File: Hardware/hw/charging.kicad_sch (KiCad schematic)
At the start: 22 parts, among them J1 Screw_Terminal_01x02, J2 Screw_Terminal_01x02, J3 Conn_01x05_Pin, J5 Conn_01x04_Pin, Q2 PMOS, Q3 PMOS, Q4 PMOS, U3 SMS3.3.TCT, U7 INA219, U8 SMS3.3.TCT

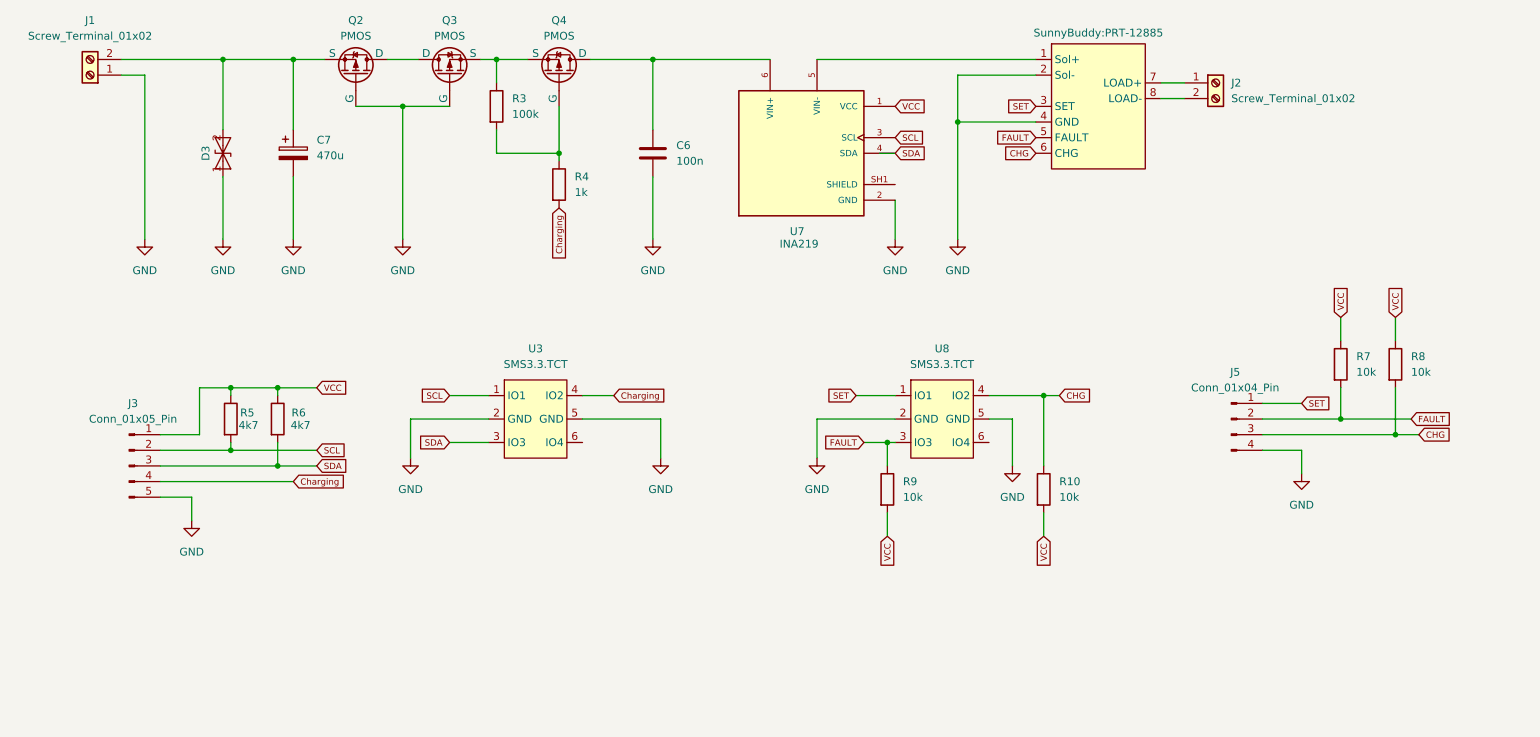
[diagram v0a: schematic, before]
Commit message: IoT board update
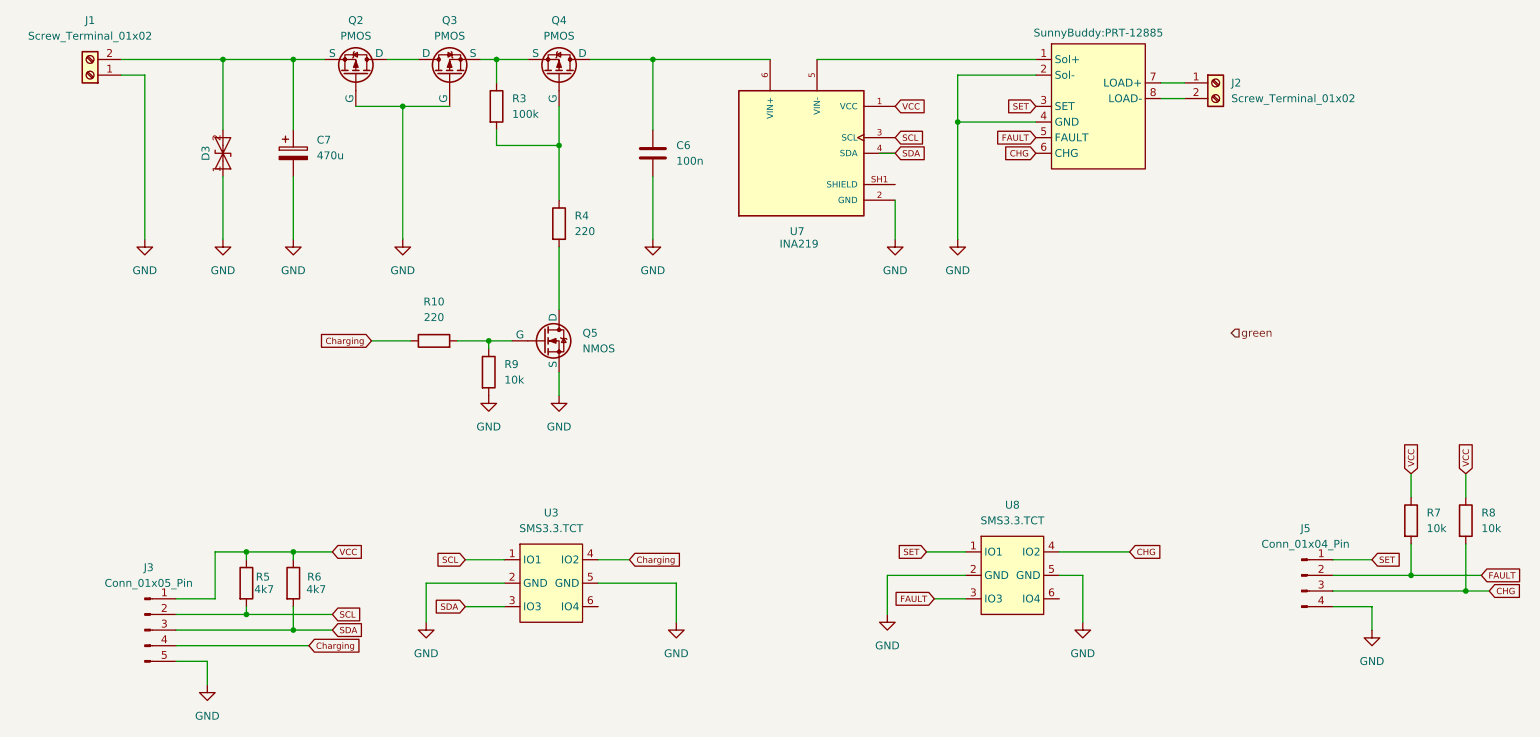
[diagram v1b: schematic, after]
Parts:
- added Q5: NMOS, symbol Simulation_SPICE:NMOS
- R10: value 10k -> 220
- R4: value 1k -> 220
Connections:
- net CHG: no longer R10.1
- net Charging: now also R10.1; no longer R4.2
- net FAULT: no longer R9.1
- net GND: now also R9.2, Q5.3 (S)
- net VCC: no longer R10.2, R9.2
- new net: Q5.1 (D), R4.2
- new net: Q5.2 (G), R10.2, R9.1
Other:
- moved on the sheet: J3, J5, R4, R5, R6, R7, R8, U3, U8
